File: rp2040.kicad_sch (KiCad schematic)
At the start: 30 parts, among them J2 USB_C_Receptacle_USB2.0, J5 Boot/Reset, U1 W25Q128JVS, U2 XC6206P332MR, U3 RP2040, Y1 12MHz

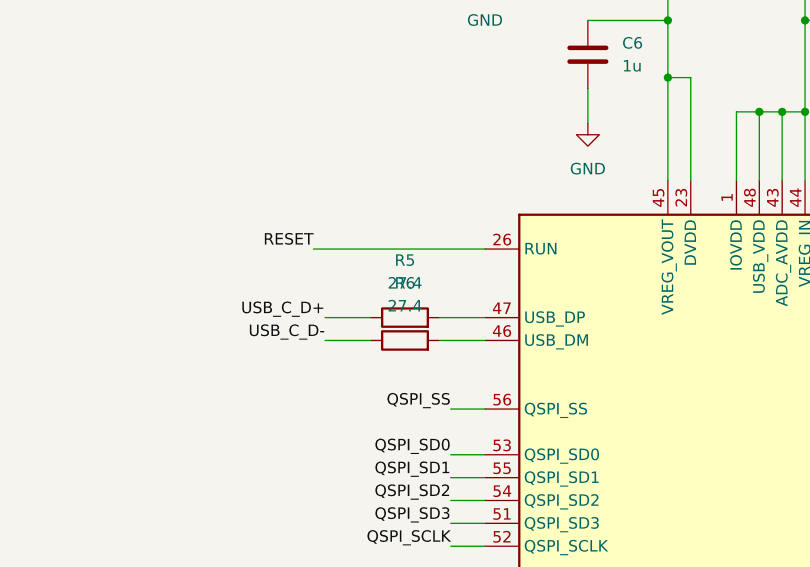
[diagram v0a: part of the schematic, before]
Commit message: JLC: Fixup for JLC Production
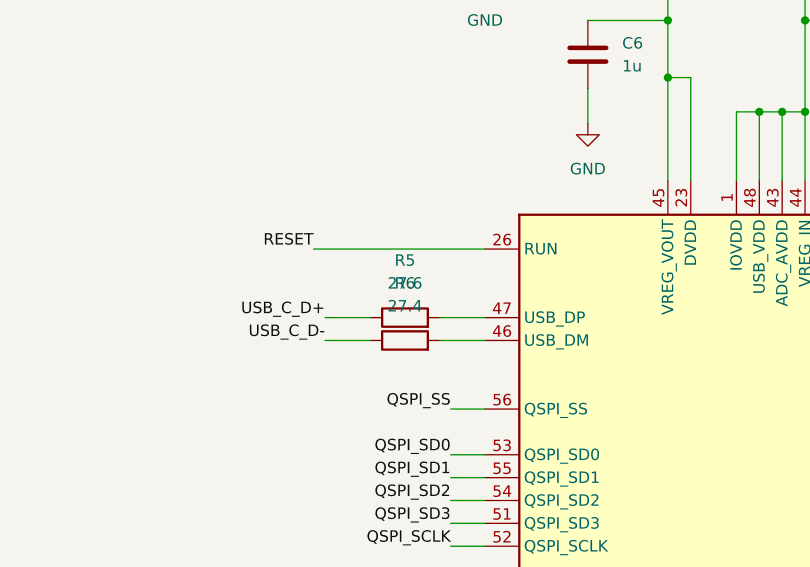
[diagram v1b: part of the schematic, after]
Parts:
- R5: value 27.4 -> 27.6; footprint Resistor_SMD:R_0201_0603Metric -> Resistor_SMD:R_1206_3216Metric; LCSC C423620 -> C333003
- R6: footprint Resistor_SMD:R_0201_0603Metric -> Resistor_SMD:R_1206_3216Metric; LCSC C423620 -> C333003
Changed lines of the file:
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@@
       (effects (font (size 1.27 1.27)))
     )
-    (property "Value" "27.4" (at 134.62 77.47 90)
-      (effects (font (size 1.27 1.27)))
-    )
-    (property "Footprint" "Resistor_SMD:R_0201_0603Metric" (at 134.62 83.058 90)
+    (property "Value" "27.6" (at 134.62 77.47 90)
+      (effects (font (size 1.27 1.27)))
+    )
+    (property "Footprint" "Resistor_SMD:R_1206_3216Metric" (at 134.62 83.058 90)
       (effects (font (size 1.27 1.27)) hide)
     )
@@
       (effects (font (size 1.27 1.27)) hide)
     )
-    (property "LCSC" "C423620" (at 134.62 81.28 90)
+    (property "LCSC" "C333003" (at 134.62 81.28 90)
       (effects (font (size 1.27 1.27)) hide)
     )
@@
       (effects (font (size 1.27 1.27)))
     )
-    (property "Footprint" "Resistor_SMD:R_0201_0603Metric" (at 134.62 85.598 90)
+    (property "Footprint" "Resistor_SMD:R_1206_3216Metric" (at 134.62 85.598 90)
       (effects (font (size 1.27 1.27)) hide)
     )
@@
       (effects (font (size 1.27 1.27)) hide)
     )
-    (property "LCSC" "C423620" (at 134.62 83.82 90)
-      (effects (font (size 1.27 1.27)) hide)
-    )
+    (property "LCSC" "C333003" (at 134.62 83.82 90)
+      (effects (font (size 1.27 1.27)) hide)
+    )
